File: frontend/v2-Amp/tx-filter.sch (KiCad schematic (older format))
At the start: 88 parts, among them K10 HK4100, K11 HK4100, K12 HK4100, K13 HK4100, K14 HK4100, K15 HK4100, K2 HK4100, K3 HK4100, K4 HK4100, K5 HK4100, K6 HK4100, K7 HK4100, K8 HK4100, K9 HK4100

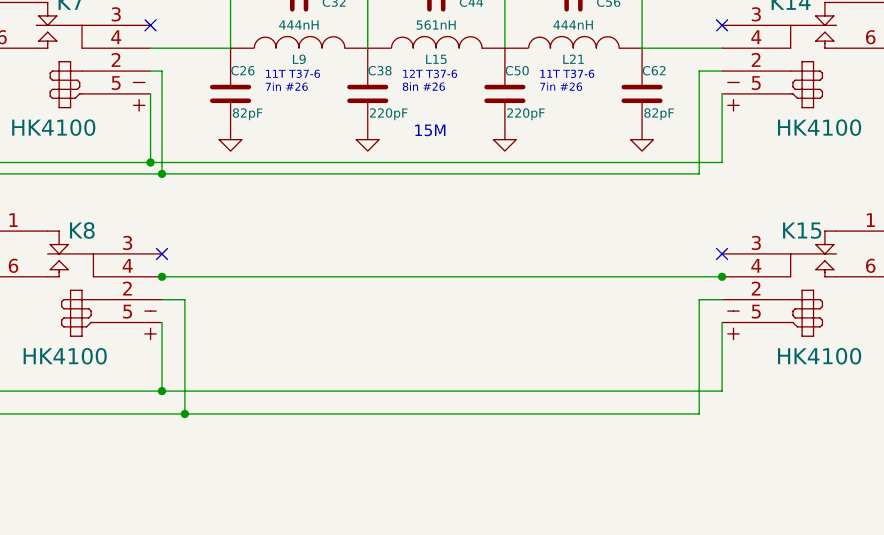
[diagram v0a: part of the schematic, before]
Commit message: Ver 1.1 changes
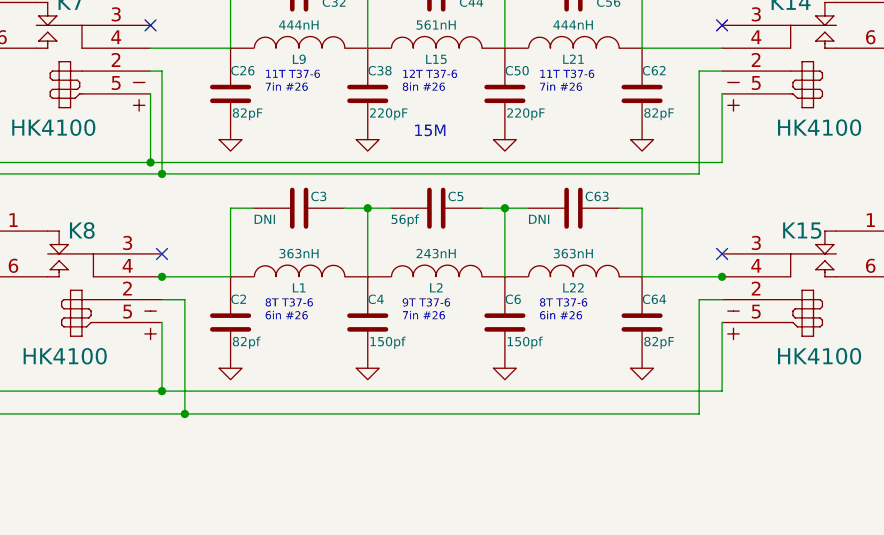
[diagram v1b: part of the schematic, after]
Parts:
- added C2: 82pf, HERMESLITE:C_0805, symbol C-RESCUE-amp
- added C3, C63: DNI, HERMESLITE:C_0805, symbol C-RESCUE-amp
- added C4, C6: 150pf, HERMESLITE:C_0805, symbol C-RESCUE-amp
- added C5: 56pf, HERMESLITE:C_0805, symbol C-RESCUE-amp
- added C64: 82pF, HERMESLITE:C_0805, symbol C-RESCUE-amp
- added L1, L22: 363nH, Resistors_SMD:R_0805_HandSoldering, symbol INDUCTOR
- added L2: 243nH, Resistors_SMD:R_0805_HandSoldering, symbol INDUCTOR
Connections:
- net GND: now also C2.2, C4.2, C6.2, C64.2
- net at K8.4: now also C2.1, C3.2, L1.1; no longer K15.4
- new net: C63.1, C64.1, K15.4, L22.2
- new net: C3.1, C4.1, C5.2, L1.2, L2.1
- new net: C5.1, C6.1, C63.2, L2.2, L22.1
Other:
- note added: "8T T37-6\n6in #26"
- note added: "9T T37-6\n7in #26"
